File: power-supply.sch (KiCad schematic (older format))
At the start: 34 parts, among them J18 Conn_01x02_Male, U11 BA33BC0FP-E2, U13 LM2990SX-5.0, U14 BA50BC0FP-E2, U15 10M08SC

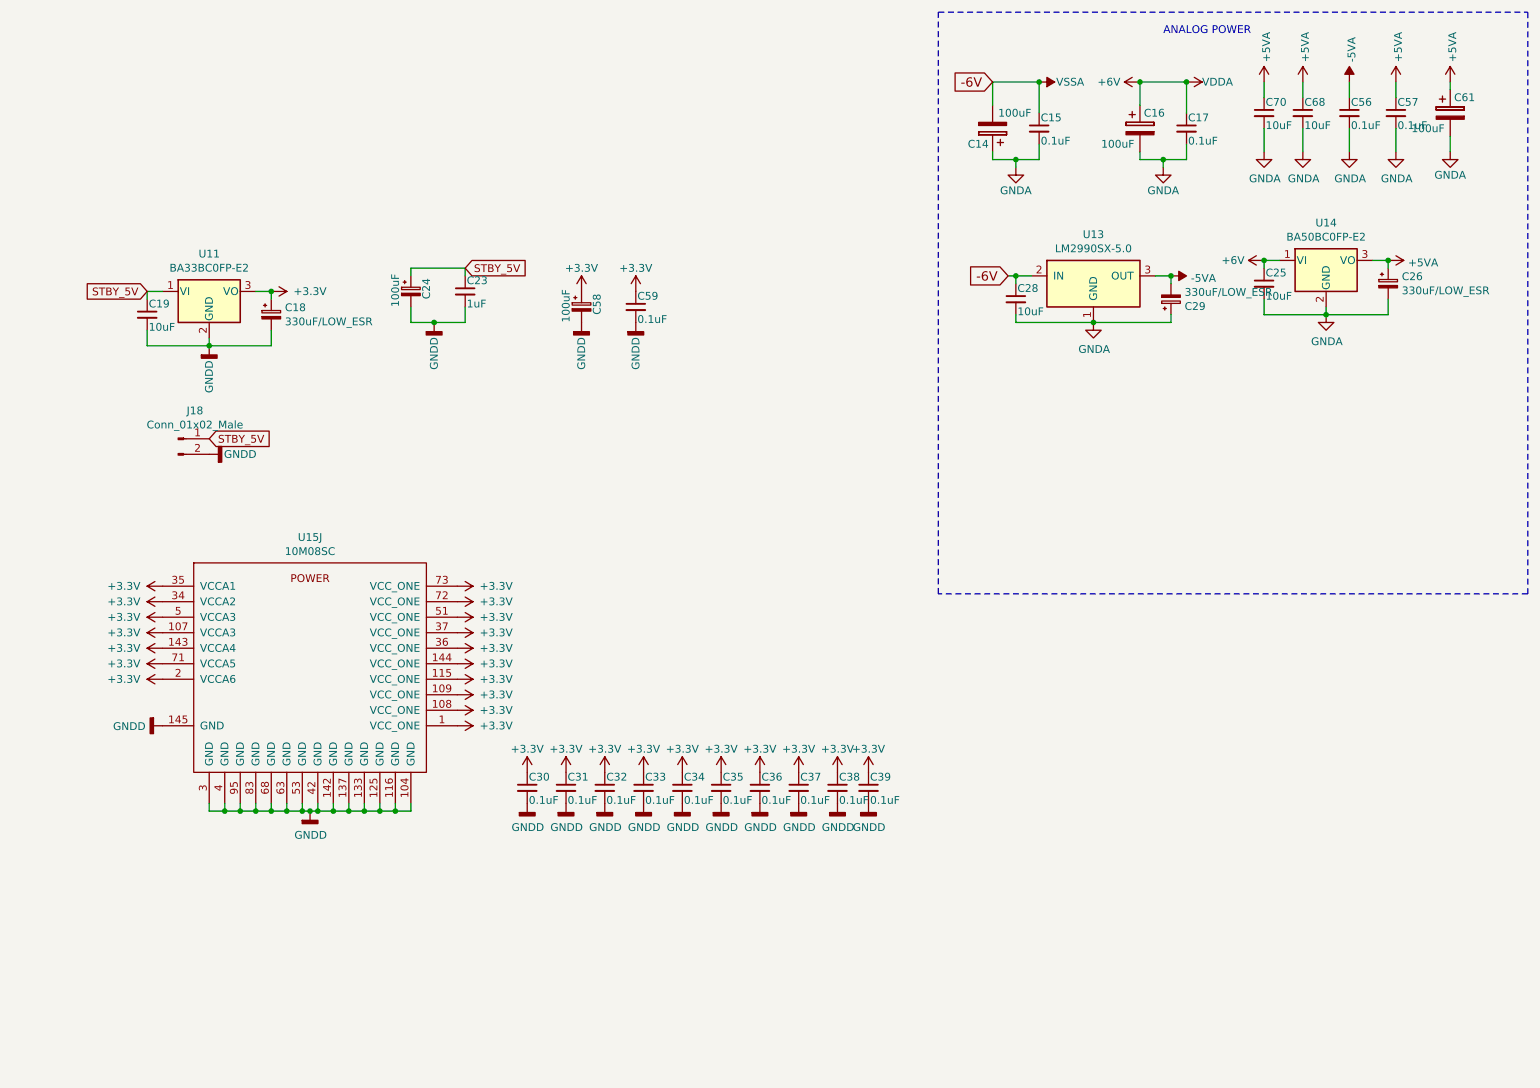
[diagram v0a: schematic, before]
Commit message: Rev. F1
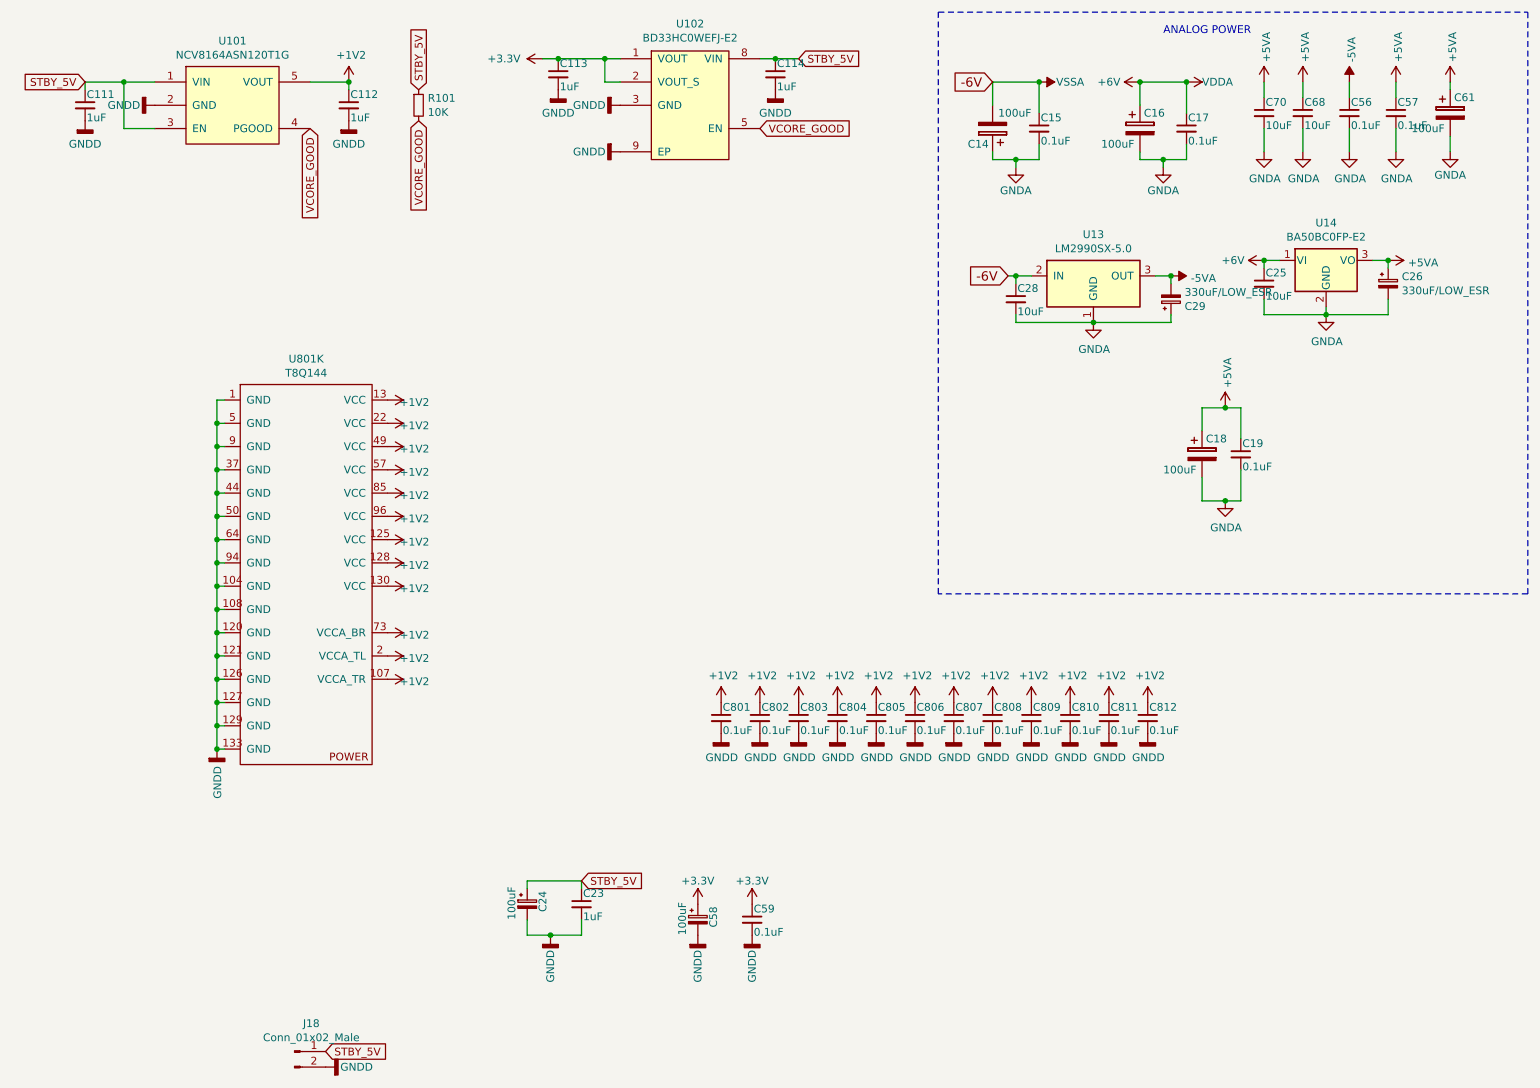
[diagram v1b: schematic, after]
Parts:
- removed C18: 330uF/LOW_ESR, Capacitor_SMD:CP_Elec_6.3x7.7, symbol Device:CP_Small
- removed U11: BA33BC0FP-E2, Package_TO_SOT_SMD:TO-252-3_TabPin2, symbol Regulator_Linear:SPX2920U-3.3_TO220
- removed U15: 10M08SC, Package_QFP:EQFP-144-1EP_20x20mm_P0.5mm_EP8.93x8.7mm_ThermalVias, symbol bkm-68x-simple-rescue:10M08SC-FPGA_Intel
- added C111, C112, C113, C114: 1uF, Capacitor_SMD:C_0805_2012Metric_Pad1.18x1.45mm_HandSolder, symbol bkm-68x-simple-rescue:C_Small
- added C18: 100uF, Capacitor_SMD:CP_Elec_6.3x5.3, symbol bkm-68x-simple-rescue:CP
- added C811, C812: 0.1uF, Capacitor_SMD:C_0603_1608Metric_Pad1.08x0.95mm_HandSolder, symbol bkm-68x-simple-rescue:C_Small
- added R101: 10K, Resistor_SMD:R_0805_2012Metric_Pad1.20x1.40mm_HandSolder, symbol Device:R_Small
- added U101: NCV8164ASN120T1G, Package_SO:TSOP-5_1.65x3.05mm_P0.95mm, symbol ldo-en-pg:NCV8164
- added U102: BD33HC0WEFJ-E2, Package_SO:HTSOP-8-1EP_3.9x4.9mm_P1.27mm_EP2.4x3.2mm_ThermalVias, symbol ldo-en-pg:BDxxHC0WEFJ
- added U801: T8Q144, Package_QFP:TQFP-144_20x20mm_P0.5mm, symbol bkm-68x-simple-rescue:T8Q144-Efinix_FPGA
- C19: value 10uF -> 0.1uF
- renumbered C30 to C801, C31 to C802, C32 to C803, C33 to C804, C34 to C805, C35 to C806, C36 to C807, C37 to C808, C38 to C809, C39 to C810
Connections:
- net +3V3: now also C113.1, U102.1 (VOUT), U102.2 (VOUT_S); no longer C801.1, C802.1, C803.1, C804.1, C805.1, C806.1, C807.1, C808.1, C809.1, C810.1
- net +5VA: now also C19.1, C18.1
- net GNDA: now also C19.2, C18.2
- net GNDD: now also C111.2, C112.2, C113.2, C114.2, C811.2, C812.2, U101.2 (GND), U102.3 (GND), U102.9 (EP), U801.1 (GND), U801.104 (GND), U801.108 (GND), U801.120 (GND), U801.121 (GND), U801.126 (GND), U801.127 (GND), U801.129 (GND), U801.133 (GND), U801.37 (GND), U801.44 (GND), U801.5 (GND), U801.50 (GND), U801.64 (GND), U801.9 (GND), U801.94 (GND); no longer C19.2
- net STBY_5V: now also C111.1, C114.1, R101.1, U101.1 (VIN), U101.3 (EN), U102.8 (VIN); no longer C19.1
- new net +1V2: C112.1, C801.1, C802.1, C803.1, C804.1, C805.1, C806.1, C807.1, C808.1, C809.1, C810.1, C811.1, C812.1, U101.5 (VOUT), U801.107 (VCCA_TR), U801.125 (VCC), U801.128 (VCC), U801.13 (VCC), U801.130 (VCC), U801.2 (VCCA_TL), U801.22 (VCC), U801.49 (VCC), U801.57 (VCC), U801.73 (VCCA_BR), U801.85 (VCC), U801.96 (VCC)
- new net VCORE_GOOD: R101.2, U101.4 (PGOOD), U102.5 (EN)
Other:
- moved on the sheet: C23, C24, C58, C59, C801, C802, C803, C804, C805, C806, C807, C808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
